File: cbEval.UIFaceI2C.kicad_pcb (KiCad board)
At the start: 2 copper layers, 140 x 108 mm, 61 parts, among them J1 Bergstik-II_1x3, J10 Bergstik-II_1x3, J11 Bergstik-II_1x3, J12 DIN41612.B.2x32.Male.Horizont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, J2 Bergstik-II_1x3, J3 Header.Hor.2x8.9-103326-0-08, J4 Header.Hor.2x8.9-103326-0-08, J5 Socket.Hor.2x8.1-5535512-8, J6 Bergstik-II_1x3, J7 Bergstik-II_1x6, J8 Bergstik-II_1x3, J9 Socket.Hor.2x8.1-5535512-8, U1 MCP23017-E/SP, U2 MCP23017-E/SP, U3 ATtiny85-20PU, U4 TN0702N3-G, U5 TN0702N3-G

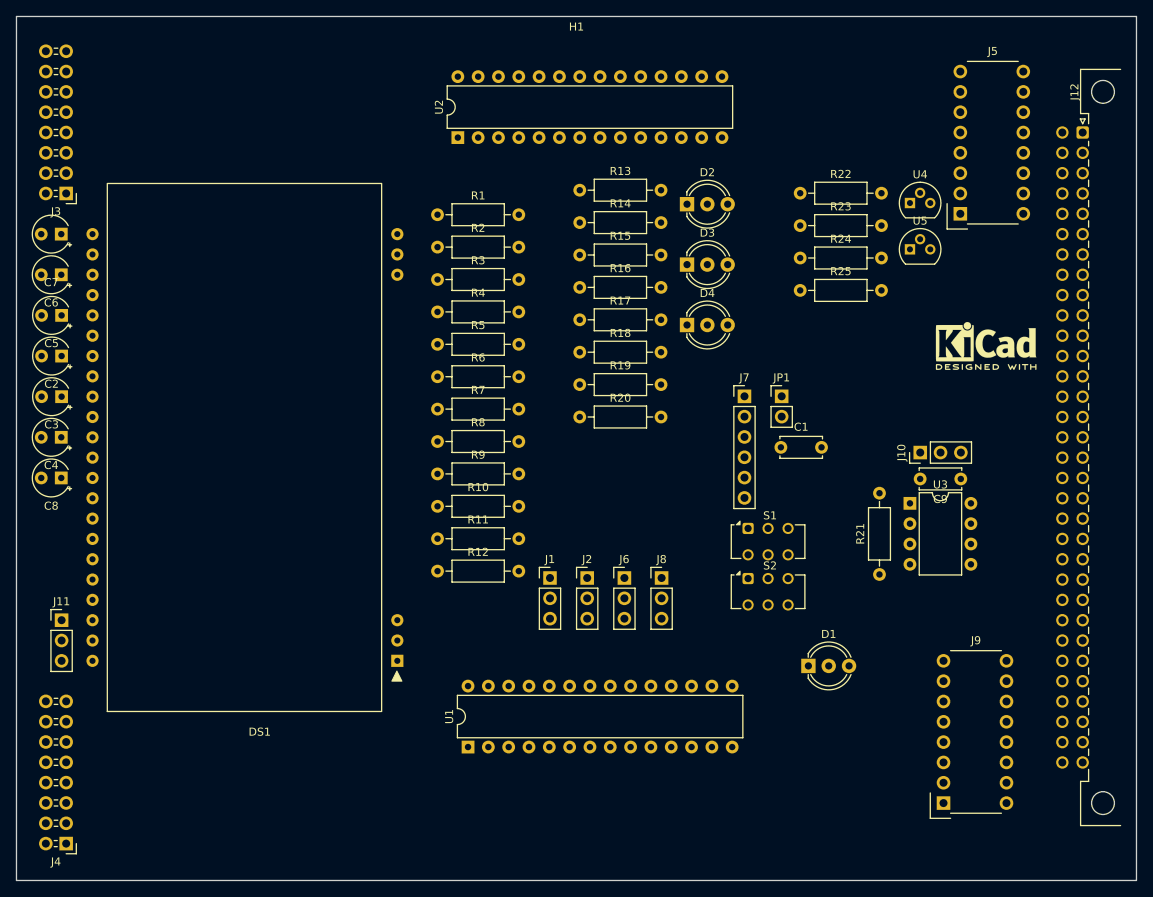
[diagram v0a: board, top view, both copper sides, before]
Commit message: Zwischenstand
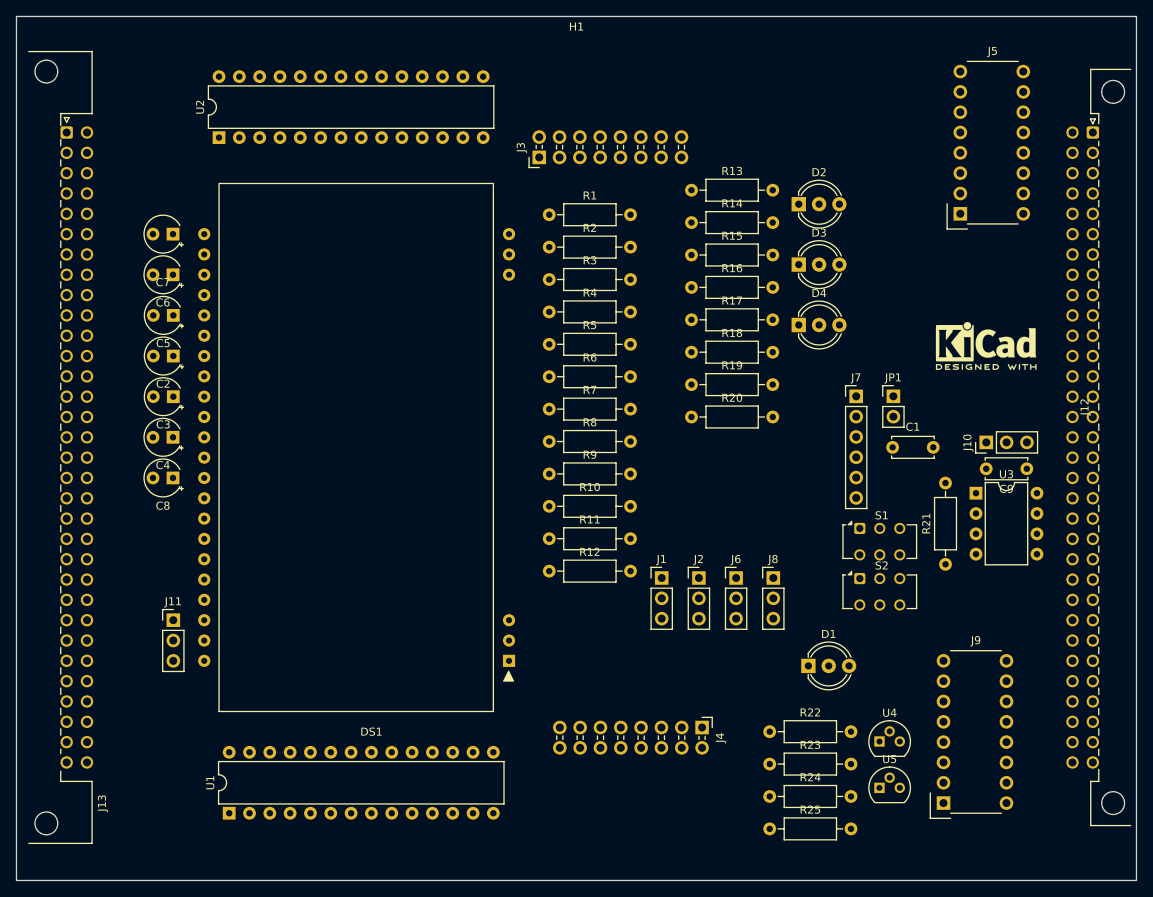
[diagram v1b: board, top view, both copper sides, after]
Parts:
- added J13: DIN41612.B.2x32.Female.Horizontal.THT, BTech.Connector.DIN41612:DIN41612.B.2x32.Female.Horizontal.THT, F.Cu at (77.5, 87.0)
- moved J4 80.8 mm to (156.9, 122.0), turned to -90 degrees
- moved R22 67.4 mm to (165.3, 122.5)
- moved R23 67.4 mm to (165.3, 126.6)
- moved R24 67.4 mm to (165.3, 130.6)
- moved U4 67.4 mm to (179.1, 123.8)
- moved U5 67.4 mm to (179.1, 129.5)
- moved R25 67.4 mm to (165.3, 134.7)
- moved J3 59.3 mm to (136.5, 50.7), turned to 90 degrees
- moved J12 39.4 mm to (205.7, 87.0)
- moved U1 31.0 mm to (97.8, 132.7)
- moved U2 29.8 mm to (96.5, 48.3)
- moved C1 14.0 mm to (180.7, 87.0)
- moved C2 14.0 mm to (90.8, 75.6)
- moved C3 14.0 mm to (90.8, 80.6)
- moved C5 14.0 mm to (90.8, 70.5)
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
